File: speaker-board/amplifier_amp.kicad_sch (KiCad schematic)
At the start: 21 parts, among them J1 Conn_01x02_Pin, U4 LM3886T_NOPB

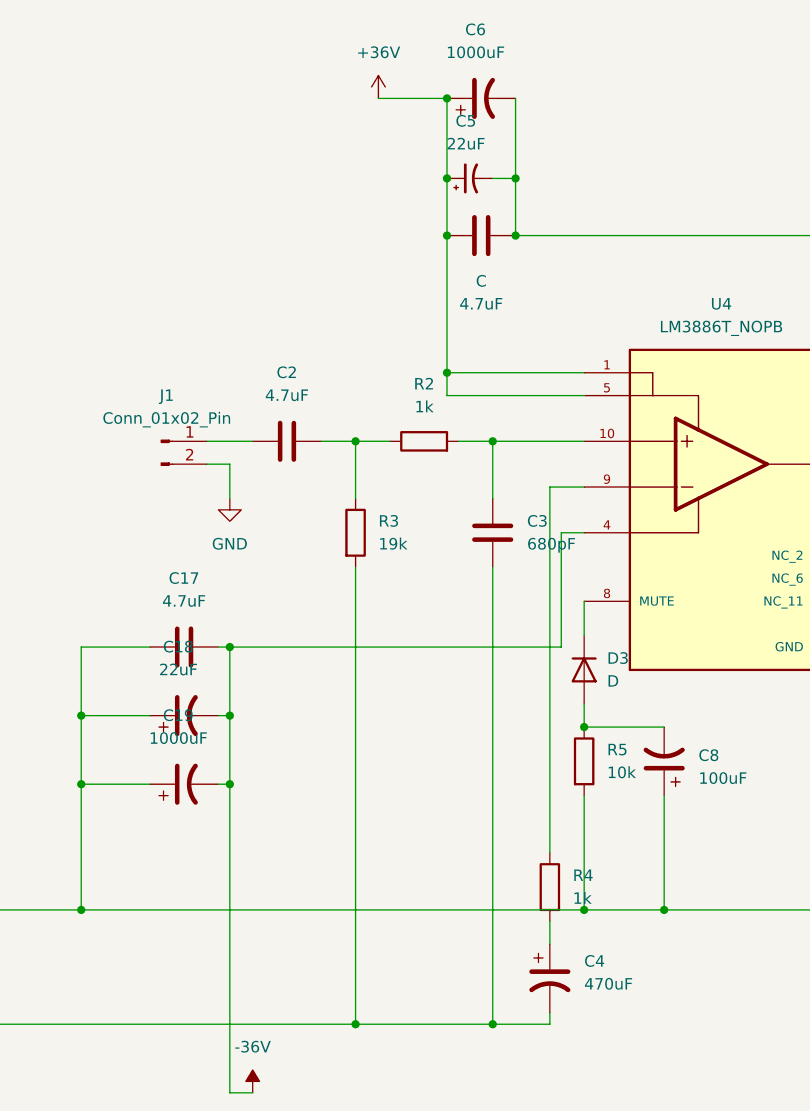
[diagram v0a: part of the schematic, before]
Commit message: update
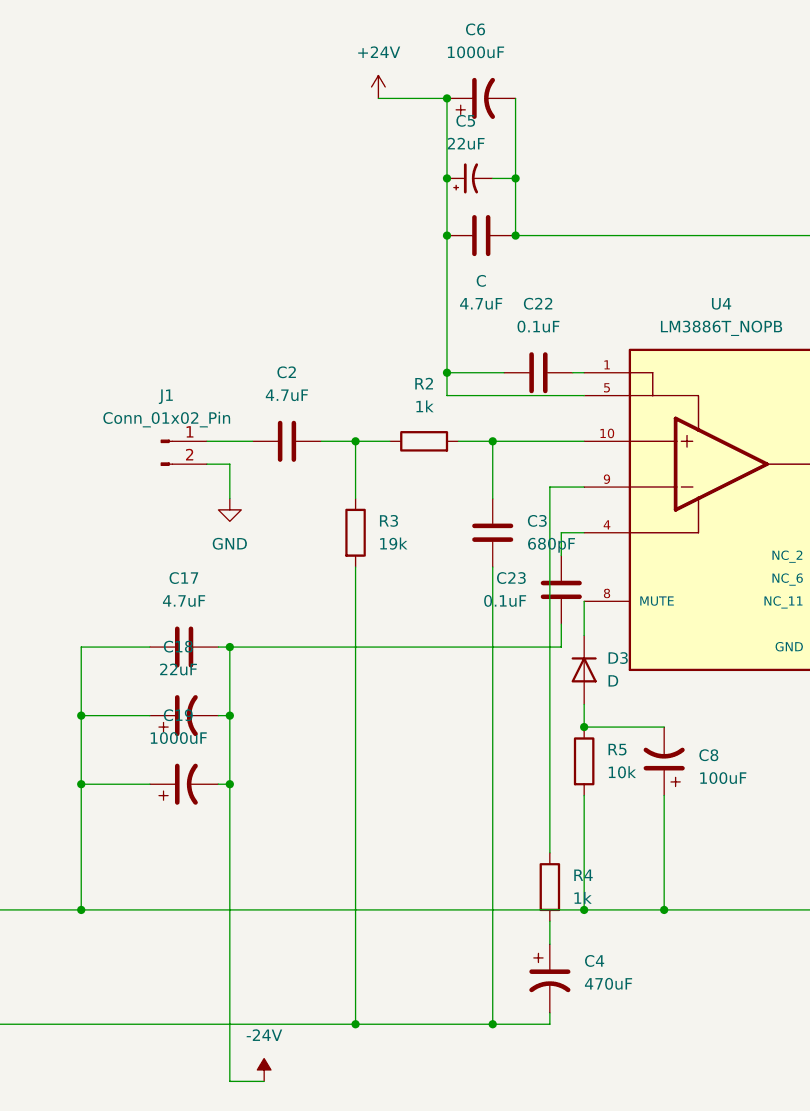
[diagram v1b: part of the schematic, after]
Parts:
- added C22, C23: 0.1uF, symbol Device:C
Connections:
- net +36V renamed +24V
- net +24V: now also C22.1; no longer U4.1
- net -36V renamed -24V
- net -24V: now also C23.2; no longer U4.4
- new net: C23.1, U4.4
- new net: C22.2, U4.1
